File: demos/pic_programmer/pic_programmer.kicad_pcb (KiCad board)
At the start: 2 copper layers, 160 x 99.1 mm, 63 parts, among them J1 DB9-FEMAL, P1 CONN_2, P101 CONN_1, P102 CONN_1, P103 CONN_1, P104 CONN_1, P105 CONN_1, P106 CONN_1, P2 SUPP28, P3 SUPP40, Q1 BC237, Q2 BC307, Q3 BC307, U1 24Cxx, U2 74HC125, U3 7805, U4 LT1373, U5 PIC_18_PINS, U6 PIC_8_PINS

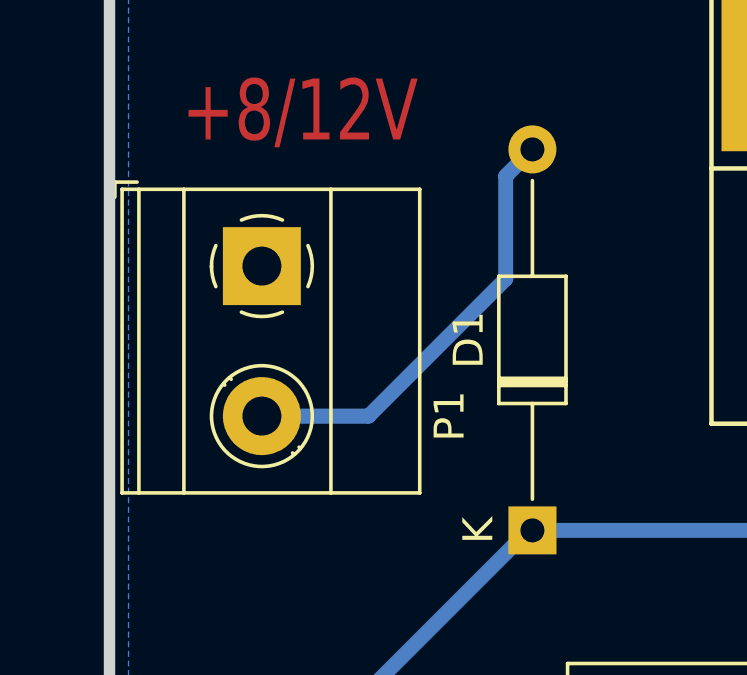
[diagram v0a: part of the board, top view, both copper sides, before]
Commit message: Update demo
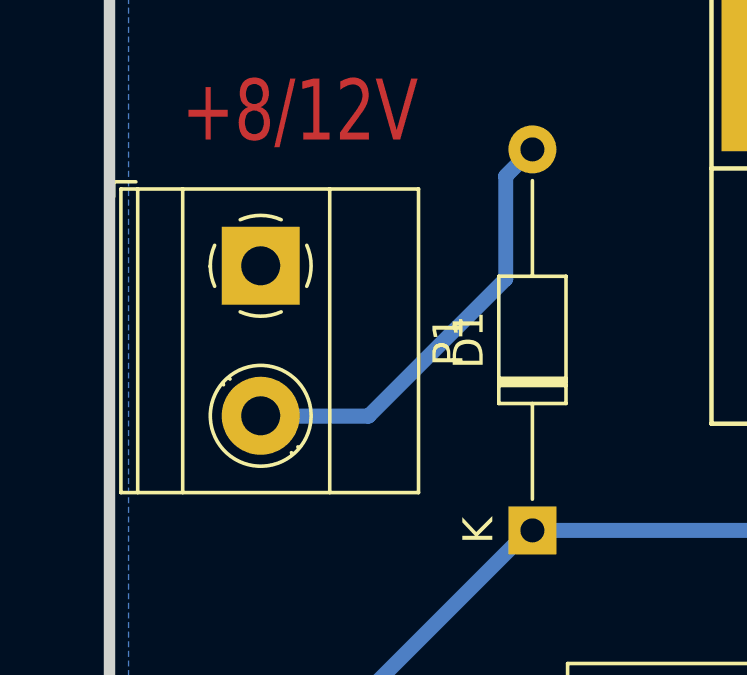
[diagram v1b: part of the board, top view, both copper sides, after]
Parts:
- C4, C5, C6, C7, C9: footprint C_Disc_D5.1mm_W3.2mm_P5.00mm -> Capacitor_THT:C_Disc_D5.1mm_W3.2mm_P5.00mm
- P3: footprint 40tex-Ell600 -> footprints:40tex-Ell600
- R1, R10, R11, R12, R13, R14, R15, R16, R17, R18, R19, R2, R20, R21, R3, R4, R5, R6, R7, R8, R9: footprint Resistors_THT:R_Axial_DIN0207_L6.3mm_D2.5mm_P10.16mm_Horizontal -> Resistor_THT:R_Axial_DIN0207_L6.3mm_D2.5mm_P10.16mm_Horizontal
- moved P1 2.51 mm to (78.7, 62.3)
